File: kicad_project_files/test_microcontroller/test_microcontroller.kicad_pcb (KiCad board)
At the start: 2 copper layers, 60 x 100 mm, 41 parts, among them J1 USB_C_Receptacle_USB2.0, SW1 SW_Push, SW2 SW_Push, SW3 SW_Push, SW4 SW_Push, SW5 SW_Push, SW6 SW_Push, SW7 SW_Push, SW8 SW_Push, SW9 SW_Push, U1 ATmega32U4-A, Y1 16mhz

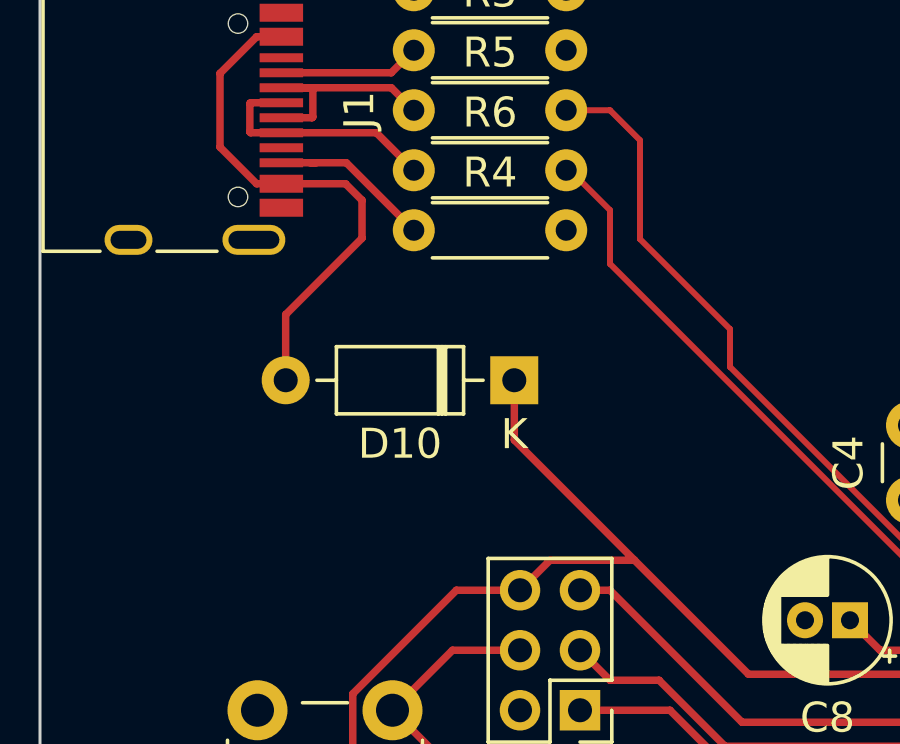
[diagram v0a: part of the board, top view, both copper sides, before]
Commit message: Revert "add diode to pcb"
This reverts commit 20722a3885263840da117607ee800e449ae5a56b.
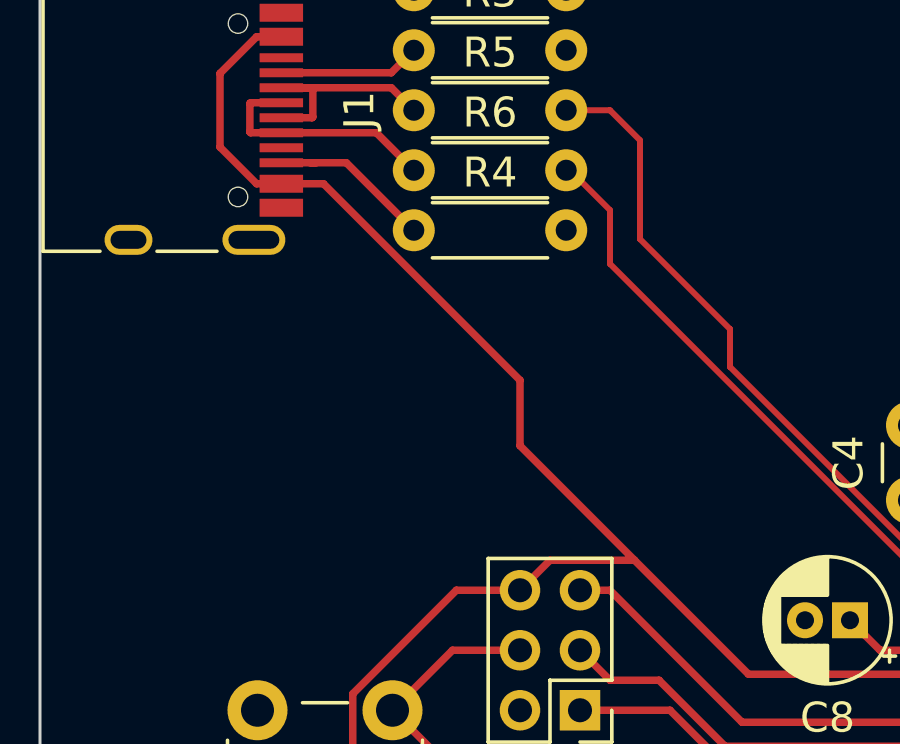
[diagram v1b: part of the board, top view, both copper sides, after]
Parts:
- removed D10: 1N4148, Diode_THT:D_DO-35_SOD27_P7.62mm_Horizontal
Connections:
- J1 pad A4: Net-(J1-PadA4) -> VCC
- J1 pad A9: Net-(J1-PadA4) -> VCC
- J1 pad B4: Net-(J1-PadA4) -> VCC
- J1 pad B9: Net-(J1-PadA4) -> VCC
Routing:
- net VCC: track 120.4 -> 138.5 mm
- net Net-(J1-PadA4): track 17.5 -> 0.00 mm
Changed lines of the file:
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@@
   (net 51 "unconnected-(U1-Pad42)")
   (net 52 "VCC")
-  (net 53 "Net-(J1-PadA4)")
   (footprint "Diode_THT:D_DO-35_SOD27_P7.62mm_Horizontal" (layer "F.Cu")
     (at 53 115.81 90)
@@
       (net 1 "GNDREF") (pinfunction "GND") (pintype "passive"))
     (pad "A4" smd rect (at -2.45 -4.045 270) (size 0.6 1.45) (layers "F.Cu" "F.Paste" "F.Mask")
-      (net 53 "Net-(J1-PadA4)") (pinfunction "VBUS") (pintype "passive"))
+      (net 52 "VCC") (pinfunction "VBUS") (pintype "passive"))
     (pad "A5" smd rect (at -1.25 -4.045 270) (size 0.3 1.45) (layers "F.Cu" "F.Paste" "F.Mask")
       (net 18 "Net-(J1-PadA5)") (pinfunction "CC1") (pintype "bidirectional"))
@@
       (net 21 "unconnected-(J1-PadA8)") (pinfunction "SBU1") (pintype "bidirectional+no_connect"))
     (pad "A9" smd rect (at 2.45 -4.045 270) (size 0.6 1.45) (layers "F.Cu" "F.Paste" "F.Mask")
-      (net 53 "Net-(J1-PadA4)") (pinfunction "VBUS") (pintype "passive"))
+      (net 52 "VCC") (pinfunction "VBUS") (pintype "passive"))
     (pad "A12" smd rect (at 3.25 -4.045 270) (size 0.6 1.45) (layers "F.Cu" "F.Paste" "F.Mask")
       (net 1 "GNDREF") (pinfunction "GND") (pintype "passive"))
@@
       (net 1 "GNDREF") (pinfunction "GND") (pintype "passive"))
     (pad "B4" smd rect (at 2.45 -4.045 270) (size 0.6 1.45) (layers "F.Cu" "F.Paste" "F.Mask")
-      (net 53 "Net-(J1-PadA4)") (pinfunction "VBUS") (pintype "passive"))
+      (net 52 "VCC") (pinfunction "VBUS") (pintype "passive"))
     (pad "B5" smd rect (at 1.75 -4.045 270) (size 0.3 1.45) (layers "F.Cu" "F.Paste" "F.Mask")
       (net 22 "Net-(J1-PadB5)") (pinfunction "CC2") (pintype "bidirectional"))
@@
       (net 23 "unconnected-(J1-PadB8)") (pinfunction "SBU2") (pintype "bidirectional+no_connect"))
     (pad "B9" smd rect (at -2.45 -4.045 270) (size 0.6 1.45) (layers "F.Cu" "F.Paste" "F.Mask")
-      (net 53 "Net-(J1-PadA4)") (pinfunction "VBUS") (pintype "passive"))
+      (net 52 "VCC") (pinfunction "VBUS") (pintype "passive"))
     (pad "B12" smd rect (at -3.25 -4.045 270) (size 0.6 1.45) (layers "F.Cu" "F.Paste" "F.Mask")
       (net 1 "GNDREF") (pinfunction "GND") (pintype "passive"))
@@
       (net 1 "GNDREF") (pintype "passive"))
     (model "${KICAD6_3DMODEL_DIR}/Capacitor_THT.3dshapes/CP_Radial_D4.0mm_P1.50mm.wrl"
-      (offset (xyz 0 0 0))
-      (scale (xyz 1 1 1))
-      (rotate (xyz 0 0 0))
-    )
-  )
-  (footprint "Diode_THT:D_DO-35_SOD27_P7.62mm_Horizontal" (layer "F.Cu")
-    (at 44.81 36 180)
-    (descr "Diode, DO-35_SOD27 series, Axial, Horizontal, pin pitch=7.62mm, , length*diameter=4*2mm^2, , http://www.diodes.com/_files/packages/DO-35.pdf")
-    (tags "Diode DO-35_SOD27 series Axial Horizontal pin pitch 7.62mm  length 4mm diameter 2mm")
-    (property "Sheetfile" "test_microcontroller.kicad_sch")
-    (property "Sheetname" "")
-    (attr through_hole)
-    (fp_text reference "D10" (at 3.81 -2.12) (layer "F.SilkS")
-      (effects (font (size 1 1) (thickness 0.15)))
-    )
-    (fp_text value "1N4148" (at 3.81 2.12) (layer "F.Fab")
-      (effects (font (size 1 1) (thickness 0.15)))
-    )
-    (fp_text user "K" (at 0 -1.8) (layer "F.SilkS")
-      (effects (font (size 1 1) (thickness 0.15)))
-    )
-    (fp_text user "K" (at 0 -1.8) (layer "F.Fab")
-      (effects (font (size 1 1) (thickness 0.15)))
-    )
-    (fp_text user "${REFERENCE}" (at 4.11 0) (layer "F.Fab")
-      (effects (font (size 0.8 0.8) (thickness 0.12)))
-    )
-    (fp_line (start 5.93 -1.12) (end 1.69 -1.12) (layer "F.SilkS") (width 0.12))
-    (fp_line (start 5.93 1.12) (end 5.93 -1.12) (layer "F.SilkS") (width 0.12))
-    (fp_line (start 1.69 1.12) (end 5.93 1.12) (layer "F.SilkS") (width 0.12))
-    (fp_line (start 1.04 0) (end 1.69 0) (layer "F.SilkS") (width 0.12))
-    (fp_line (start 2.41 -1.12) (end 2.41 1.12) (layer "F.SilkS") (width 0.12))
-    (fp_line (start 2.29 -1.12) (end 2.29 1.12) (layer "F.SilkS") (width 0.12))
-    (fp_line (start 1.69 -1.12) (end 1.69 1.12) (layer "F.SilkS") (width 0.12))
-    (fp_line (start 2.53 -1.12) (end 2.53 1.12) (layer "F.SilkS") (width 0.12))
-    (fp_line (start 6.58 0) (end 5.93 0) (layer "F.SilkS") (width 0.12))
-    (fp_line (start -1.05 1.25) (end 8.67 1.25) (layer "F.CrtYd") (width 0.05))
-    (fp_line (start 8.67 -1.25) (end -1.05 -1.25) (layer "F.CrtYd") (width 0.05))
-    (fp_line (start 8.67 1.25) (end 8.67 -1.25) (layer "F.CrtYd") (width 0.05))
-    (fp_line (start -1.05 -1.25) (end -1.05 1.25) (layer "F.CrtYd") (width 0.05))
-    (fp_line (start 5.81 1) (end 5.81 -1) (layer "F.Fab") (width 0.1))
-    (fp_line (start 2.51 -1) (end 2.51 1) (layer "F.Fab") (width 0.1))
-    (fp_line (start 5.81 -1) (end 1.81 -1) (layer "F.Fab") (width 0.1))
-    (fp_line (start 1.81 1) (end 5.81 1) (layer "F.Fab") (width 0.1))
-    (fp_line (start 2.31 -1) (end 2.31 1) (layer "F.Fab") (width 0.1))
-    (fp_line (start 7.62 0) (end 5.81 0) (layer "F.Fab") (width 0.1))
-    (fp_line (start 2.41 -1) (end 2.41 1) (layer "F.Fab") (width 0.1))
-    (fp_line (start 0 0) (end 1.81 0) (layer "F.Fab") (width 0.1))
-    (fp_line (start 1.81 -1) (end 1.81 1) (layer "F.Fab") (width 0.1))
-    (pad "1" thru_hole rect (at 0 0 180) (size 1.6 1.6) (drill 0.8) (layers *.Cu *.Mask)
-      (net 52 "VCC") (pinfunction "K") (pintype "passive"))
-    (pad "2" thru_hole oval (at 7.62 0 180) (size 1.6 1.6) (drill 0.8) (layers *.Cu *.Mask)
-      (net 53 "Net-(J1-PadA4)") (pinfunction "A") (pintype "passive"))
-    (model "${KICAD6_3DMODEL_DIR}/Diode_THT.3dshapes/D_DO-35_SOD27_P7.62mm_Horizontal.wrl"
       (offset (xyz 0 0 0))
       (scale (xyz 1 1 1))
@@
   (segment (start 61.3 48.2) (end 51.835718 48.2) (width 0.25) (layer "F.Cu") (net 36))
   (segment (start 64.6 50.7) (end 64.6 47.4) (width 0.25) (layer "F.Cu") (net 52))
-  (segment (start 44.81 37.992141) (end 44.81 36) (width 0.25) (layer "F.Cu") (net 52))
+  (segment (start 45 38.182141) (end 45 36) (width 0.25) (layer "F.Cu") (net 52))
+  (segment (start 37.045 29.45) (end 36.220978 29.45) (width 0.25) (layer "F.Cu") (net 52))
+  (segment (start 48.818348 42.000489) (end 45 38.182141) (width 0.25) (layer "F.Cu") (net 52))
   (segment (start 61.3 41.8) (end 59.8 41.8) (width 0.25) (layer "F.Cu") (net 52))
+  (segment (start 45 36) (end 38.45 29.45) (width 0.25) (layer "F.Cu") (net 52))
   (segment (start 39.425489 48.425489) (end 46.54 55.54) (width 0.25) (layer "F.Cu") (net 52))
   (segment (start 67 44.3) (end 70.925489 40.374511) (width 0.25) (layer "F.Cu") (net 52))
@@
   (segment (start 70.2 48.2) (end 67 45) (width 0.25) (layer "F.Cu") (net 52))
   (segment (start 71 40.3) (end 70.925489 40.374511) (width 0.25) (layer "F.Cu") (net 52))
+  (segment (start 36.220978 24.55) (end 37.045 24.55) (width 0.25) (layer "F.Cu") (net 52))
   (segment (start 77 50) (end 75.2 48.2) (width 0.25) (layer "F.Cu") (net 52))
   (segment (start 67 45) (end 67 44.3) (width 0.25) (layer "F.Cu") (net 52))
   (segment (start 62.3 41.8) (end 63.374511 40.725489) (width 0.25) (layer "F.Cu") (net 52))
-  (segment (start 48.818348 42.000489) (end 44.81 37.992141) (width 0.25) (layer "F.Cu") (net 52))
   (segment (start 64.6 51.7) (end 62.3 54) (width 0.25) (layer "F.Cu") (net 52))
   (segment (start 71 39.3) (end 71 40.3) (width 0.25) (layer "F.Cu") (net 52))
   (segment (start 62 35) (end 62 38.3) (width 0.25) (layer "F.Cu") (net 52))
   (segment (start 39.425489 46.451368) (end 39.425489 48.425489) (width 0.25) (layer "F.Cu") (net 52))
+  (segment (start 35 28.229022) (end 35 25.770978) (width 0.25) (layer "F.Cu") (net 52))
   (segment (start 42.876857 43) (end 39.425489 46.451368) (width 0.25) (layer "F.Cu") (net 52))
   (segment (start 62 38.3) (end 63 39.3) (width 0.25) (layer "F.Cu") (net 52))
@@
   (segment (start 64.6 50.7) (end 64.6 51.7) (width 0.25) (layer "F.Cu") (net 52))
   (segment (start 46.54 55.54) (end 46.54 59) (width 0.25) (layer "F.Cu") (net 52))
+  (segment (start 35 25.770978) (end 36.220978 24.55) (width 0.25) (layer "F.Cu") (net 52))
   (segment (start 62.3 54) (end 59 54) (width 0.25) (layer "F.Cu") (net 52))
   (segment (start 61.3 41.8) (end 62.3 41.8) (width 0.25) (layer "F.Cu") (net 52))
@@
   (segment (start 64.6 47.4) (end 67 45) (width 0.25) (layer "F.Cu") (net 52))
   (segment (start 72 35) (end 72 38.3) (width 0.25) (layer "F.Cu") (net 52))
+  (segment (start 38.45 29.45) (end 37.045 29.45) (width 0.25) (layer "F.Cu") (net 52))
   (segment (start 45 43) (end 42.876857 43) (width 0.25) (layer "F.Cu") (net 52))
+  (segment (start 36.220978 29.45) (end 35 28.229022) (width 0.25) (layer "F.Cu") (net 52))
   (segment (start 72.7 48.2) (end 70.2 48.2) (width 0.25) (layer "F.Cu") (net 52))
-  (segment (start 37.045 29.45) (end 36.220978 29.45) (width 0.25) (layer "F.Cu") (net 53))
-  (segment (start 39.734511 30) (end 39.184511 29.45) (width 0.25) (layer "F.Cu") (net 53))
-  (segment (start 39.734511 31.265489) (end 39.734511 30) (width 0.25) (layer "F.Cu") (net 53))
-  (segment (start 36.220978 24.55) (end 37.045 24.55) (width 0.25) (layer "F.Cu") (net 53))
-  (segment (start 35 28.229022) (end 35 25.770978) (width 0.25) (layer "F.Cu") (net 53))
-  (segment (start 37.19 33.81) (end 39.734511 31.265489) (width 0.25) (layer "F.Cu") (net 53))
-  (segment (start 39.184511 29.45) (end 37.045 29.45) (width 0.25) (layer "F.Cu") (net 53))
-  (segment (start 35 25.770978) (end 36.220978 24.55) (width 0.25) (layer "F.Cu") (net 53))
-  (segment (start 37.19 36) (end 37.19 33.81) (width 0.25) (layer "F.Cu") (net 53))
-  (segment (start 36.220978 29.45) (end 35 28.229022) (width 0.25) (layer "F.Cu") (net 53))
   (zone (net 1) (net_name "GNDREF") (layer "F.Cu") (hatch edge 0.508)
     (connect_pads (clearance 0.3))
